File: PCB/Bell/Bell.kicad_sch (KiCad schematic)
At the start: 31 parts, among them J1 USB-C, J2 POWER, J3 Conn_01x08, J5 Conn_01x05, J6 Conn_01x02, J8 Shelly, U1 MD8942, U10 ESP32-S3-MINI-1, U3 ISL89410, U4 ISL89410, U7 AA, U8 QR

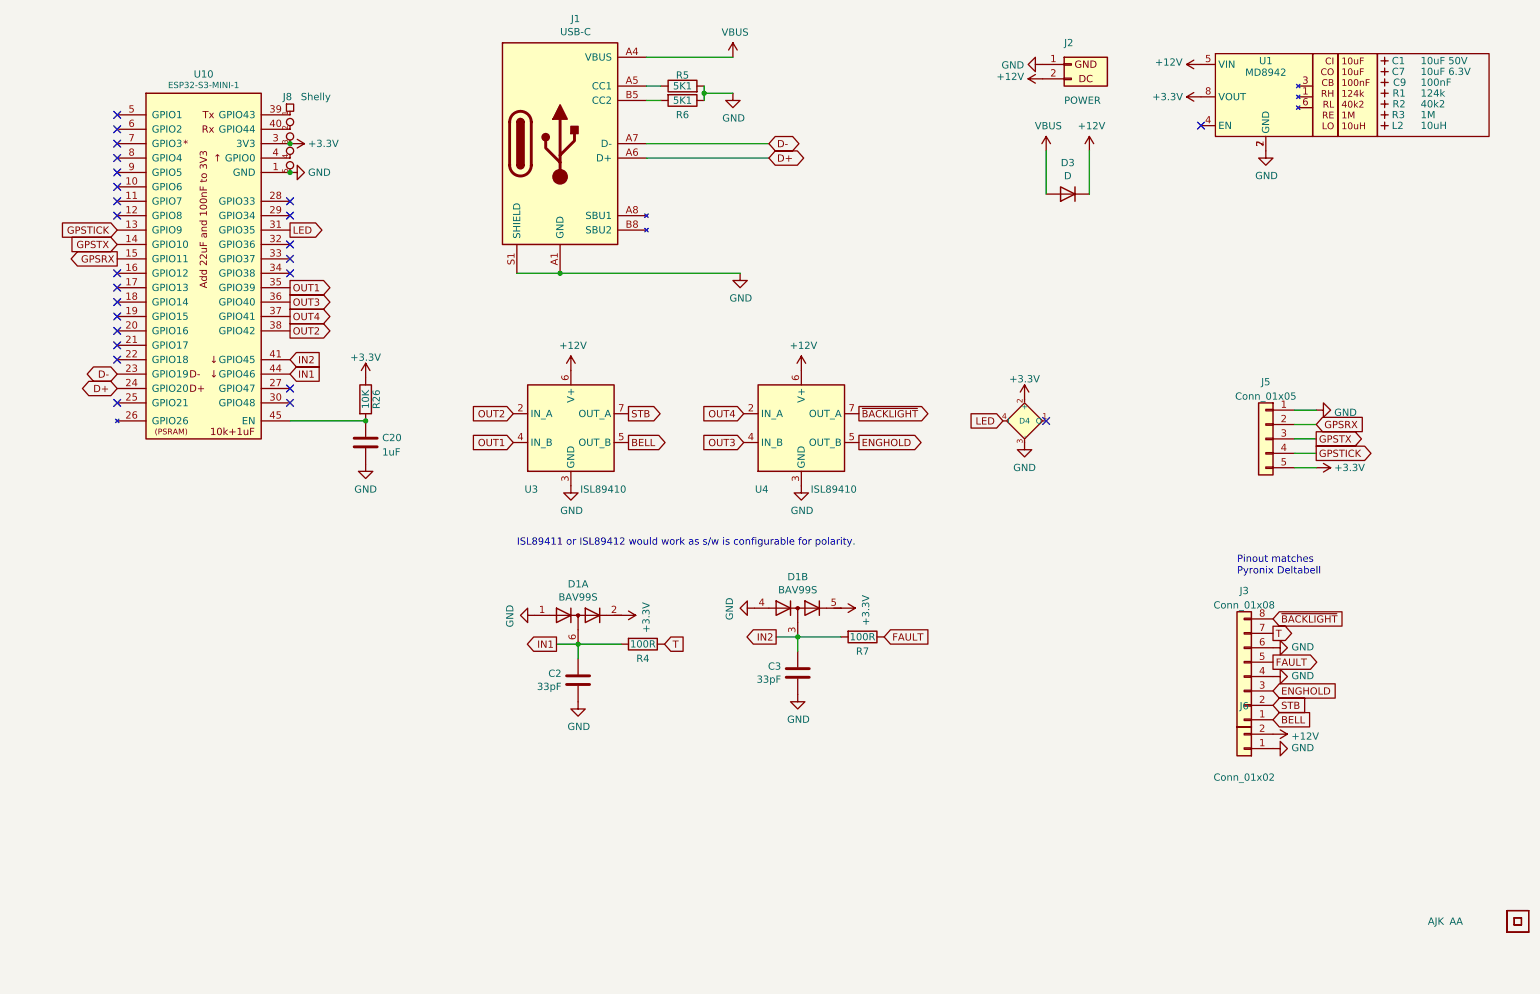
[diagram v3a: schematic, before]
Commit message: LEDs
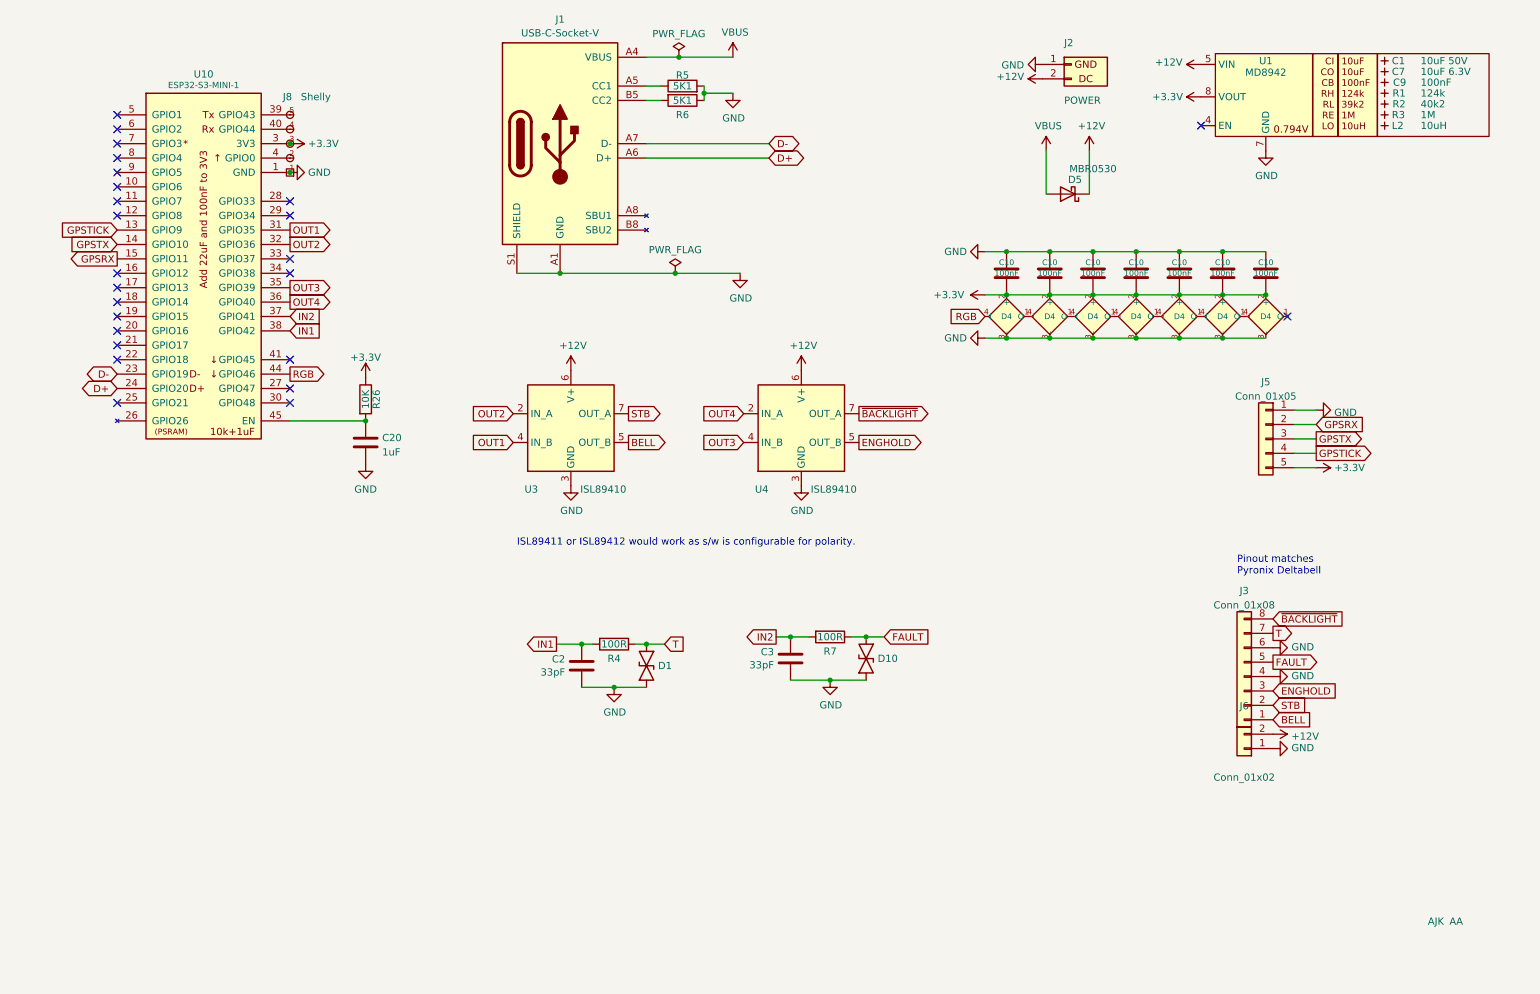
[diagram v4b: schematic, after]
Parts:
- removed D1: BAV99S, RevK:SOT-363_SC-70-6, symbol Diode:BAV99S
- removed D3: D, RevK:D_1206, symbol Device:D
- removed J1: USB-C, RevK:USC16-TR, symbol RevK:USB-C
- removed U8: QR, RevK:QR-SS, symbol RevK:QR
- added C10 (x7): 100nF, RevK:C_0402, symbol Device:C
- added D1, D10: ~, RevK:DFN1006-2L, symbol RevK:ES05D1MC10
- added D4 (x6): XL-1010RGBC-WS2812B, RevK:SMD1010, symbol RevK:WS2812B-1mm
- added D5: MBR0530, RevK:D_SOD-123, symbol Diode:1N5819
- added J1: USB-C-Socket-V, RevK:USB-C-Socket-H, symbol RevK:USB-C-Socket-H
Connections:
- net +12V: now also D5.1 (K)
- net D+: now also J1.A6 (D+), J1.B6 (D+)
- net D-: now also J1.A7 (D-), J1.B7 (D-)
- net FAULT: now also D10.1
- net GND: now also J8.1 (GND), C10.1, C10.1, C10.1, C10.1, C10.1, C10.1, C10.1, D1.2, D10.2, D4.3 (-), D4.3 (-), D4.3 (-), D4.3 (-), D4.3 (-), D4.3 (-), J1.A1 (GND), J1.A12 (GND), J1.B1 (GND), J1.B12 (GND), J1.S1 (SHIELD); no longer J8.5 (Tx)
- net IN1: now also U10.38 (GPIO42); no longer U10.44 (GPIO46)
- net IN2: now also U10.37 (GPIO41); no longer U10.41 (GPIO45)
- net OUT1: now also U10.31 (GPIO35); no longer U10.35 (GPIO39)
- net OUT2: now also U10.32 (GPIO36); no longer U10.38 (GPIO42)
- net OUT3: now also U10.35 (GPIO39); no longer U10.36 (GPIO40)
- net OUT4: now also U10.36 (GPIO40); no longer U10.37 (GPIO41)
- net T: now also D1.1
- net VBUS: now also D5.2 (A), J1.A4 (VBUS), J1.A9 (VBUS), J1.B4 (VBUS), J1.B9 (VBUS)
- net at R5.1: now also J1.A5 (CC1)
- net at R6.2: now also J1.B5 (CC2)
- net at U10.39 (GPIO43): now also J8.5 (Tx); no longer J8.1 (GND)
- net at U10.4 (GPIO0): now also J8.2 (0); no longer J8.4 (Rx)
- net at U10.40 (GPIO44): now also J8.4 (Rx); no longer J8.2 (0)
- net at D4.1 (O): now also D4.4 (I)
- net +3V3 renamed +3.3V
- net +3.3V: now also C10.2, C10.2, C10.2, C10.2, C10.2, C10.2, C10.2, D4.2 (+), D4.2 (+), D4.2 (+), D4.2 (+), D4.2 (+), D4.2 (+)
- net LED renamed RGB
- net RGB: now also U10.44 (GPIO46); no longer U10.31 (GPIO35)
- new net: D4.1 (O), D4.4 (I) (x5)
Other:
- moved on the sheet: C2, C3, D4, J8, R4, R7
